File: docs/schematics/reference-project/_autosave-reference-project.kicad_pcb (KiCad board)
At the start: 2 copper layers, 38 x 68 mm, 23 parts, among them J1 UART, Q1 MMBT3904, SW1 INPUT_0, SW2 INPUT_1, SW3 INPUT_2, SW4 INPUT_3, SW5 INPUT_4, SW6 INPUT_5, SW7 RESET, U1 74HC165D, U2 ATTINY85-20PU

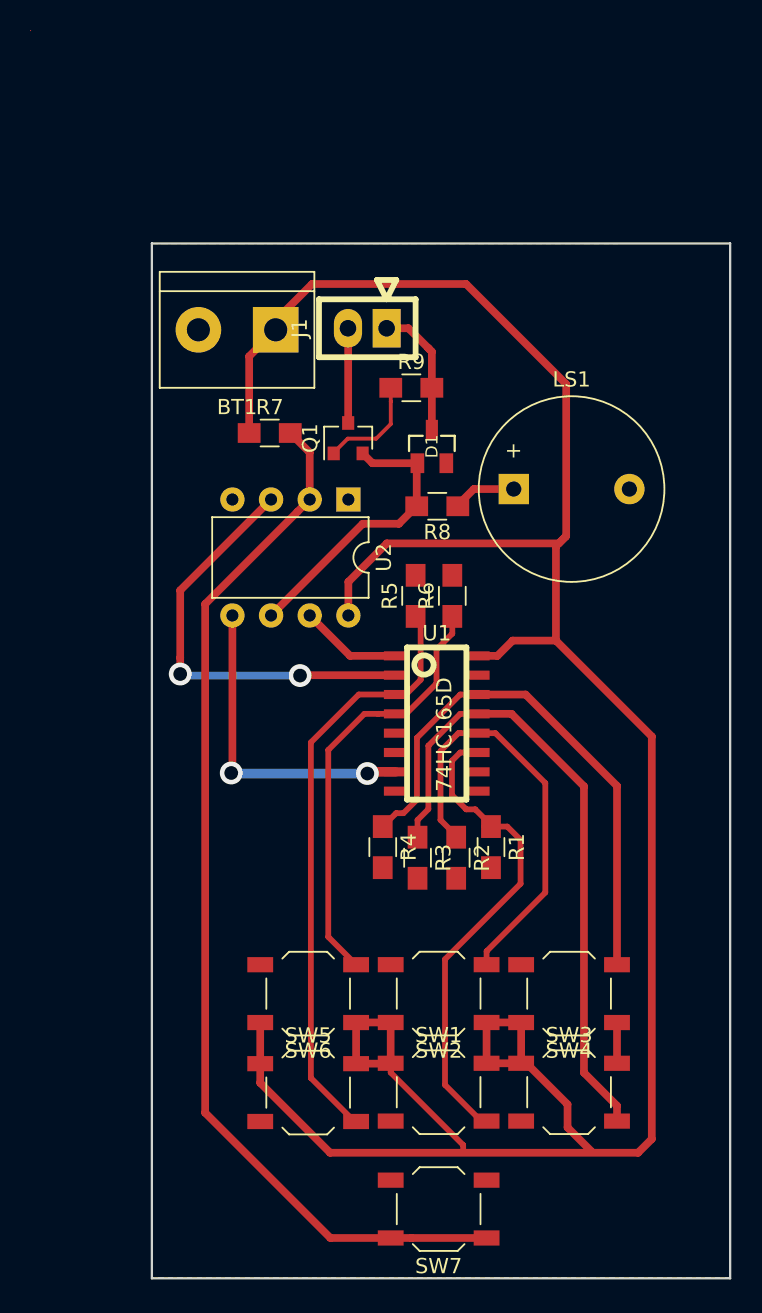
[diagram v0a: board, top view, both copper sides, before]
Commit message: Updated to v2.
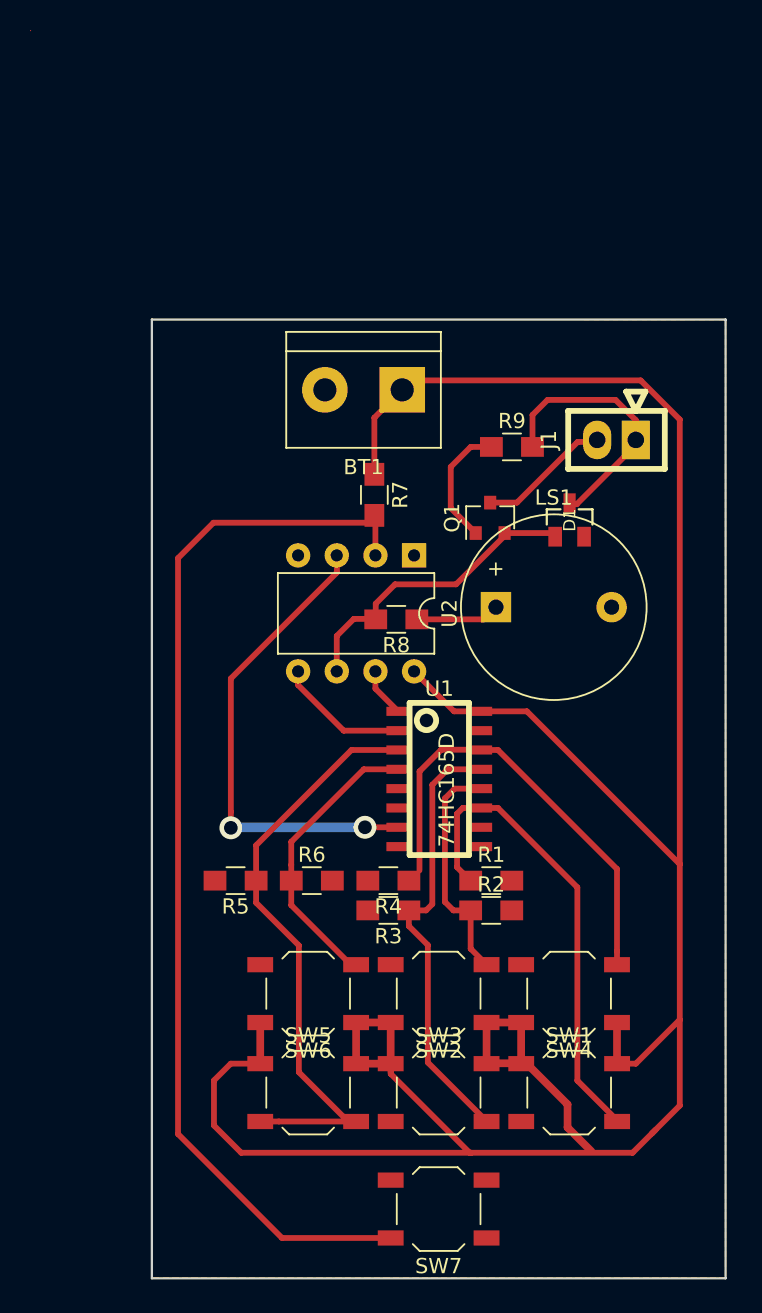
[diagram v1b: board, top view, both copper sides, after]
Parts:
- moved R5 22.1 mm to (50.5, 98.9), turned to 180 degrees
- moved R6 20.9 mm to (55.5, 98.9), turned to 0 degrees
- moved J1 17.9 mm to (75.5, 69.9)
- moved Q1 10.7 mm to (67.2, 75.0)
- moved D1 10.3 mm to (72.5, 75.2)
- moved BT1 9.20 mm to (61.5, 66.6)
- moved SW1 8.58 mm to (72.4, 112.8)
- moved SW3 8.57 mm to (63.8, 112.8)
- moved R7 7.99 mm to (59.6, 73.5), turned to 270 degrees
- moved R8 7.90 mm to (61.1, 81.7)
- moved LS1 7.85 mm to (67.6, 80.9)
- moved R9 7.67 mm to (68.7, 70.4)
- moved U2 5.67 mm to (62.2, 77.5)
- moved R2 4.15 mm to (67.3, 100.8), turned to 0 degrees
- moved R3 3.96 mm to (60.5, 100.8), turned to 180 degrees
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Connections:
- U2 pad 3: Net-(U1-Pad2) -> Net-(U1-Pad7)
- U2 pad 5: Net-(U1-Pad7) -> Net-(U1-Pad2)
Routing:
- net Net-(U1-Pad2): track 28.1 -> 8.72 mm, vias 2 -> 0
- net Net-(R3-Pad1): track 42.3 -> 29.1 mm
- net Net-(R2-Pad1): track 28.4 -> 15.5 mm
- net Net-(U1-Pad7): track 21.2 -> 31.7 mm
- net Net-(R6-Pad1): track 29.1 -> 19.0 mm
- net Net-(D1-Pad3): track 8.87 -> 17.5 mm
- net Net-(R4-Pad1): track 36.1 -> 29.6 mm
- net +3V3: track 176.4 -> 180.7 mm
- net Net-(U1-Pad1): track 6.75 -> 3.25 mm
- net Net-(J1-Pad2): track 6.28 -> 8.78 mm
- net Net-(D1-Pad1): track 19.2 -> 20.9 mm
- net Net-(R7-Pad2): track 69.9 -> 71.3 mm
- net Net-(LS1-Pad1): track 4.19 -> 5.55 mm
- net Net-(Q1-Pad1): track 6.96 -> 8.24 mm
- net Net-(R1-Pad1): track 32.3 -> 31.5 mm
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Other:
- board size 38 x 68 mm -> 37.7 x 63 mm

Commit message: Updated to v3.
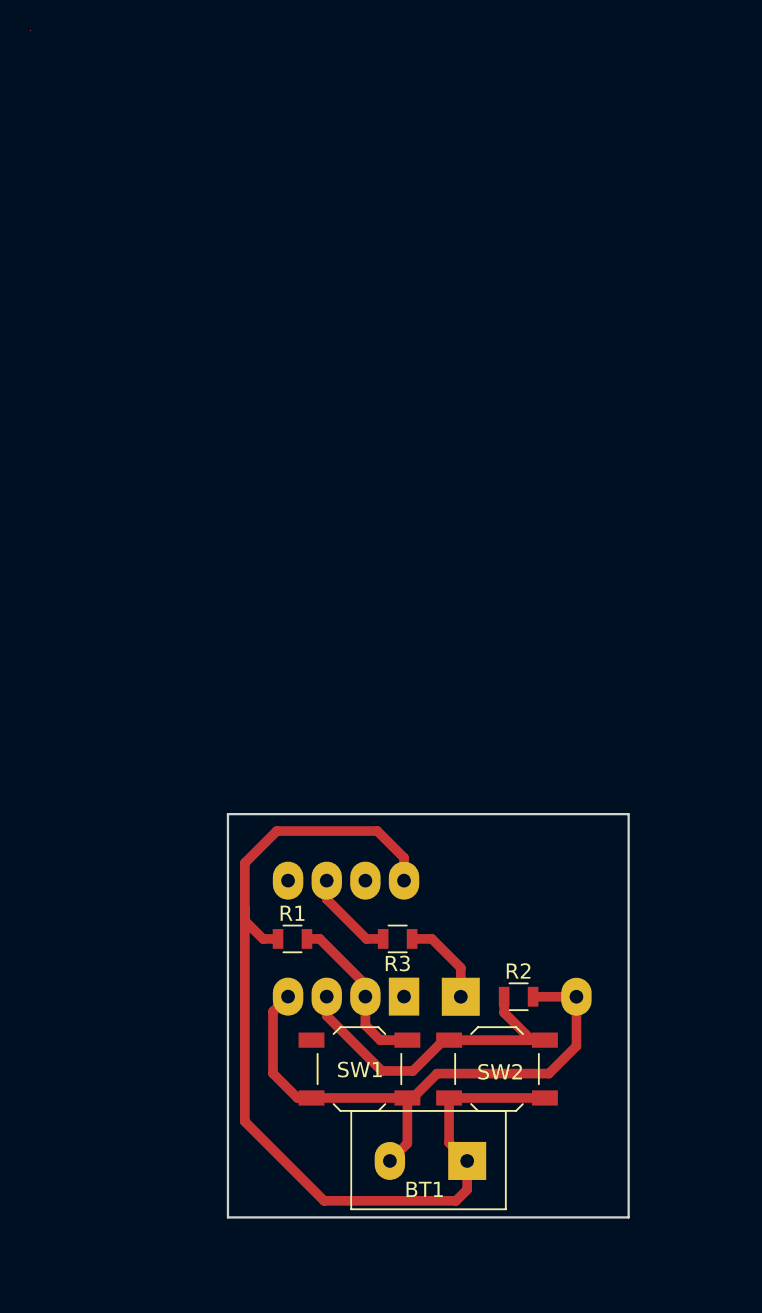
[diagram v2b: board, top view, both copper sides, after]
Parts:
- removed D1: BAT54C, smd-semi:SOT-23
- removed J1: UART, footprints:Header_2_Pin
- removed Q1: MMBT3904, TO_SOT_Packages_SMD:SOT-23
- removed R4, R5, R6, R7, R9: 10K, Resistors_SMD:R_0805_HandSoldering
- removed R8: 220, Resistors_SMD:R_0805_HandSoldering
- removed SW3: INPUT_2, Buttons_Switches_SMD:SW_SPST_TL3342
- removed SW4: INPUT_3, Buttons_Switches_SMD:SW_SPST_TL3342
- removed SW5: INPUT_4, Buttons_Switches_SMD:SW_SPST_TL3342
- removed SW6: INPUT_5, Buttons_Switches_SMD:SW_SPST_TL3342
- removed SW7: RESET, Buttons_Switches_SMD:SW_SPST_TL3342
- removed U2: ATTINY85-20PU, Housings_DIP:DIP-8_W7.62mm
- BT1: footprint Connectors:bornier2 -> reference-project-footprints:bornier2
- LS1: footprint Buzzers_Beepers:Buzzer_12x9.5RM7.6 -> reference-project-footprints:Buzzer_12x9.5RM7.6; moved to B.Cu
- R1, R2: footprint Resistors_SMD:R_0805_HandSoldering -> Resistors_SMD:R_0805
- R3: value 10K -> 220; footprint Resistors_SMD:R_0805_HandSoldering -> Resistors_SMD:R_0805
- SW1: value INPUT_0 -> RESET
- SW2: value INPUT_1 -> INPUT_5
- U1: value 74HC165D -> ATTINY85-20PU; footprint footprints:SOIC_16_0.154IN -> reference-project-footprints:DIP-8_W7.62mm; moved to B.Cu
- moved BT1 50.2 mm to (65.7, 116.7)
- moved LS1 25.7 mm to (65.3, 106.5)
- moved U1 15.1 mm to (61.6, 106.5), turned to 90 degrees
- moved SW1 13.9 mm to (58.6, 111.2), turned to 180 degrees
- moved R1 13.6 mm to (54.2, 102.7)
- moved SW2 6.27 mm to (67.7, 111.2), turned to 0 degrees
- moved R2 5.95 mm to (69.1, 106.5)
- moved R3 1.97 mm to (61.1, 102.7)
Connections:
- R1 pad 1: Net-(R1-Pad1) -> +3V3
- R1 pad 2: GND -> Net-(R1-Pad2)
- R3 pad 1: Net-(R3-Pad1) -> Net-(LS1-Pad1)
- R3 pad 2: GND -> Net-(R3-Pad2)
- SW1 pad 1: +3V3 -> GND
- SW1 pad 2: Net-(R1-Pad1) -> Net-(R1-Pad2)
- SW2 pad 1: +3V3 -> Net-(R2-Pad1)
- SW2 pad 2: Net-(R2-Pad1) -> +3V3
- U1 pad 1: Net-(U1-Pad1) -> (no net)
- U1 pad 2: Net-(U1-Pad2) -> Net-(R1-Pad2)
- U1 pad 3: Net-(R5-Pad1) -> Net-(R2-Pad1)
- U1 pad 4: Net-(R6-Pad1) -> GND
- U1 pad 5: GND -> (no net)
- U1 pad 6: GND -> Net-(R3-Pad2)
- U1 pad 7: Net-(U1-Pad7) -> (no net)
- U1 pad 8: GND -> +3V3
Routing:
- net +3V3: track 180.7 -> 64.0 mm
- net Net-(R7-Pad2): track 71.3 -> 0.00 mm
- net Net-(R5-Pad1): track 39.4 -> 0.00 mm
- net GND: track 0.00 -> 38.3 mm
- net Net-(U1-Pad7): track 31.7 -> 0.00 mm, vias 2 -> 0
- net Net-(R1-Pad1): track 31.5 -> 0.00 mm
- net Net-(R4-Pad1): track 29.6 -> 0.00 mm
- net Net-(R3-Pad1): track 29.1 -> 0.00 mm
- net Net-(D1-Pad1): track 20.9 -> 0.00 mm
- net Net-(R6-Pad1): track 19.0 -> 0.00 mm
- net Net-(D1-Pad3): track 17.5 -> 0.00 mm
- net Net-(R1-Pad2): track 0.00 -> 10.9 mm
- net Net-(J1-Pad2): track 8.78 -> 0.00 mm
- net Net-(U1-Pad2): track 8.72 -> 0.00 mm
- net Net-(Q1-Pad1): track 8.24 -> 0.00 mm
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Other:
- board size 37.7 x 63 mm -> 26.3 x 26.5 mm
- net class Default: clearance 0.3 -> 0.4
- rule trace_clearance: 0.3 -> 0.4
